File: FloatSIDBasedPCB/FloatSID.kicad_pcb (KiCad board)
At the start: 2 copper layers, 22 x 66.5 mm, 18 parts, among them M1 Motor_DC, SW1 SW, SW2 Limit Switch, U2 MS583730BA01-50, U4 XiaoESP32C3

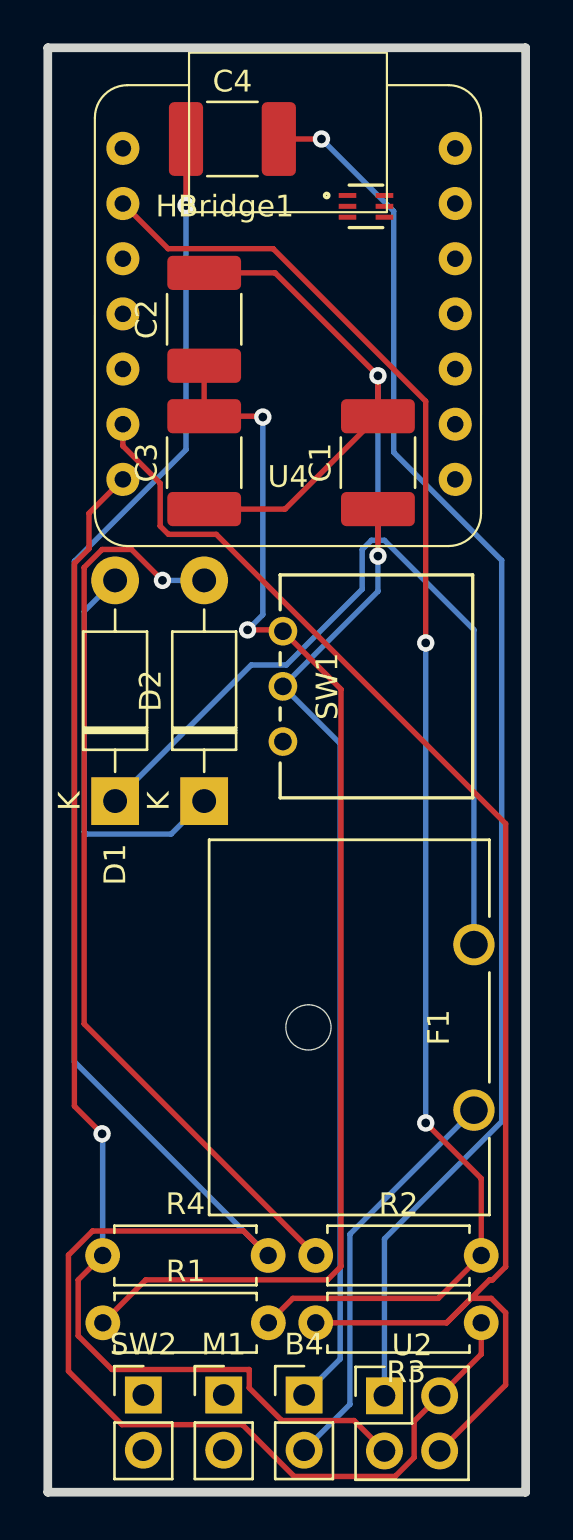
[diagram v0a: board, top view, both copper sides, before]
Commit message: Updated PCB
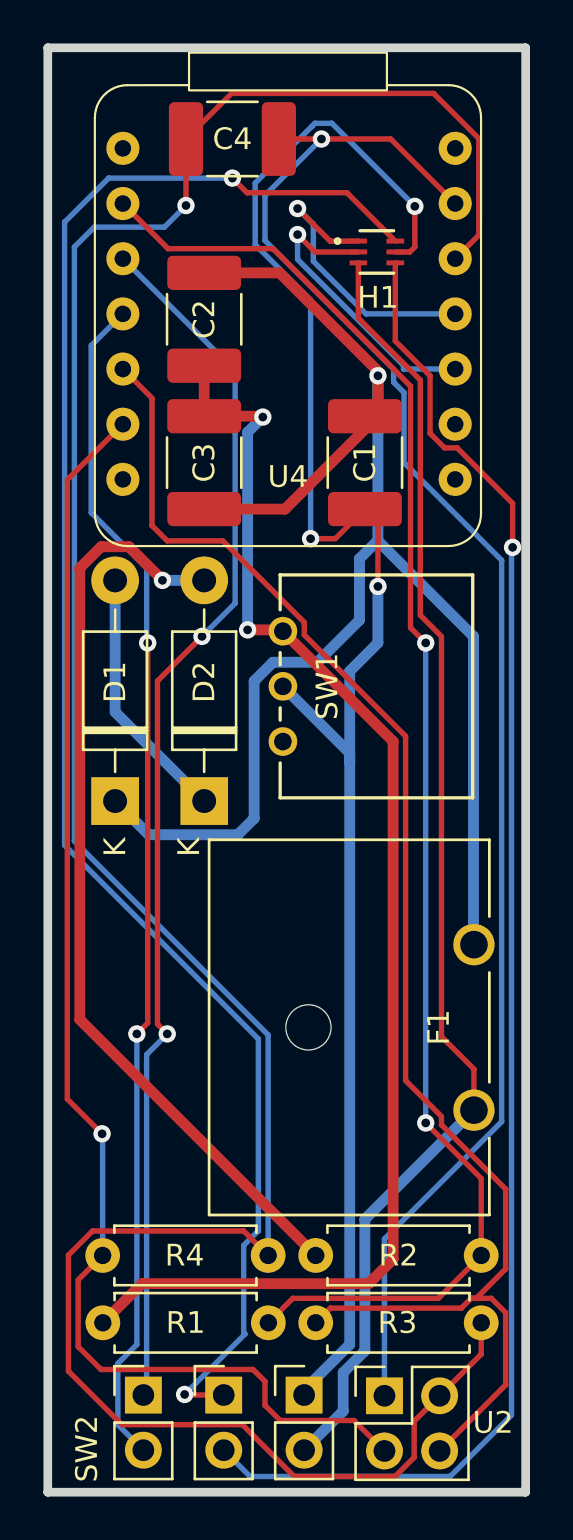
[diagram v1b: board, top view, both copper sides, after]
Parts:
- moved H1 2.16 mm to (129.6, 82.6)
- moved C1 0.60 mm to (129.1, 92.3)
- renumbered HBridge1 to H1
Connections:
- H1 pad 1: (no net) -> Net-(HBridge1-In1)
- H1 pad 2: (no net) -> unconnected-(U4-D8-Pad9)
- H1 pad 3: (no net) -> Net-(B4--)
- H1 pad 4: (no net) -> Net-(HBridge1-Out2)
- H1 pad 5: (no net) -> Net-(B4-+)
- H1 pad 6: (no net) -> Net-(HBridge1-Out1)
- SW2 pad 1: (no net) -> unconnected-(U4-D1-Pad2)
- SW2 pad 2: (no net) -> unconnected-(U4-D2-Pad3)
- U4 pad 3V3: (no net) -> Net-(U2-VDD)
- U4 pad 4: unconnected-(U4-D3-Pad4) -> Net-(U2-SDA)
- U4 pad 5: Net-(U2-SDA) -> Net-(U2-SCL)
- U4 pad 6: Net-(U2-SCL) -> (no net)
- U4 pad GND: (no net) -> Net-(U2-GND)
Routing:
- net Net-(HBridge1-Out1): track 0.00 -> 78.2 mm, vias 0 -> 2
- net Net-(HBridge1-Out2): track 0.00 -> 70.6 mm, vias 0 -> 1
- net unconnected-(U4-D1-Pad2): track 0.00 -> 56.6 mm, vias 0 -> 2
- net unconnected-(U4-D2-Pad3): track 0.00 -> 55.2 mm, vias 0 -> 2
- net Net-(B4--): track 18.9 -> 60.1 mm
- net Net-(B4-+): track 44.4 -> 80.5 mm, vias 1 -> 3
- net Net-(U2-VDD): track 98.5 -> 121.5 mm
- net unconnected-(U4-D8-Pad9): track 0.00 -> 13.7 mm, vias 0 -> 1
- net Net-(HBridge1-In1): track 0.00 -> 13.7 mm, vias 0 -> 1
- net Net-(U2-GND): track 65.5 -> 75.0 mm
- net Net-(D1-A): track 18.4 -> 11.9 mm
- net Net-(D1-K): track 67.9 -> 73.5 mm
- net Net-(U2-SCL): track 58.2 -> 61.4 mm
- net Net-(HBridge1-VDD): track 59.2 -> 62.4 mm
- net Net-(U2-SDA): track 68.3 -> 69.5 mm
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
